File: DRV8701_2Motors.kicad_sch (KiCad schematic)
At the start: 24 parts, among them J1 Conn_01x02, J2 Conn_01x10, J3 Conn_01x10, SW1 SW_SPDT_321

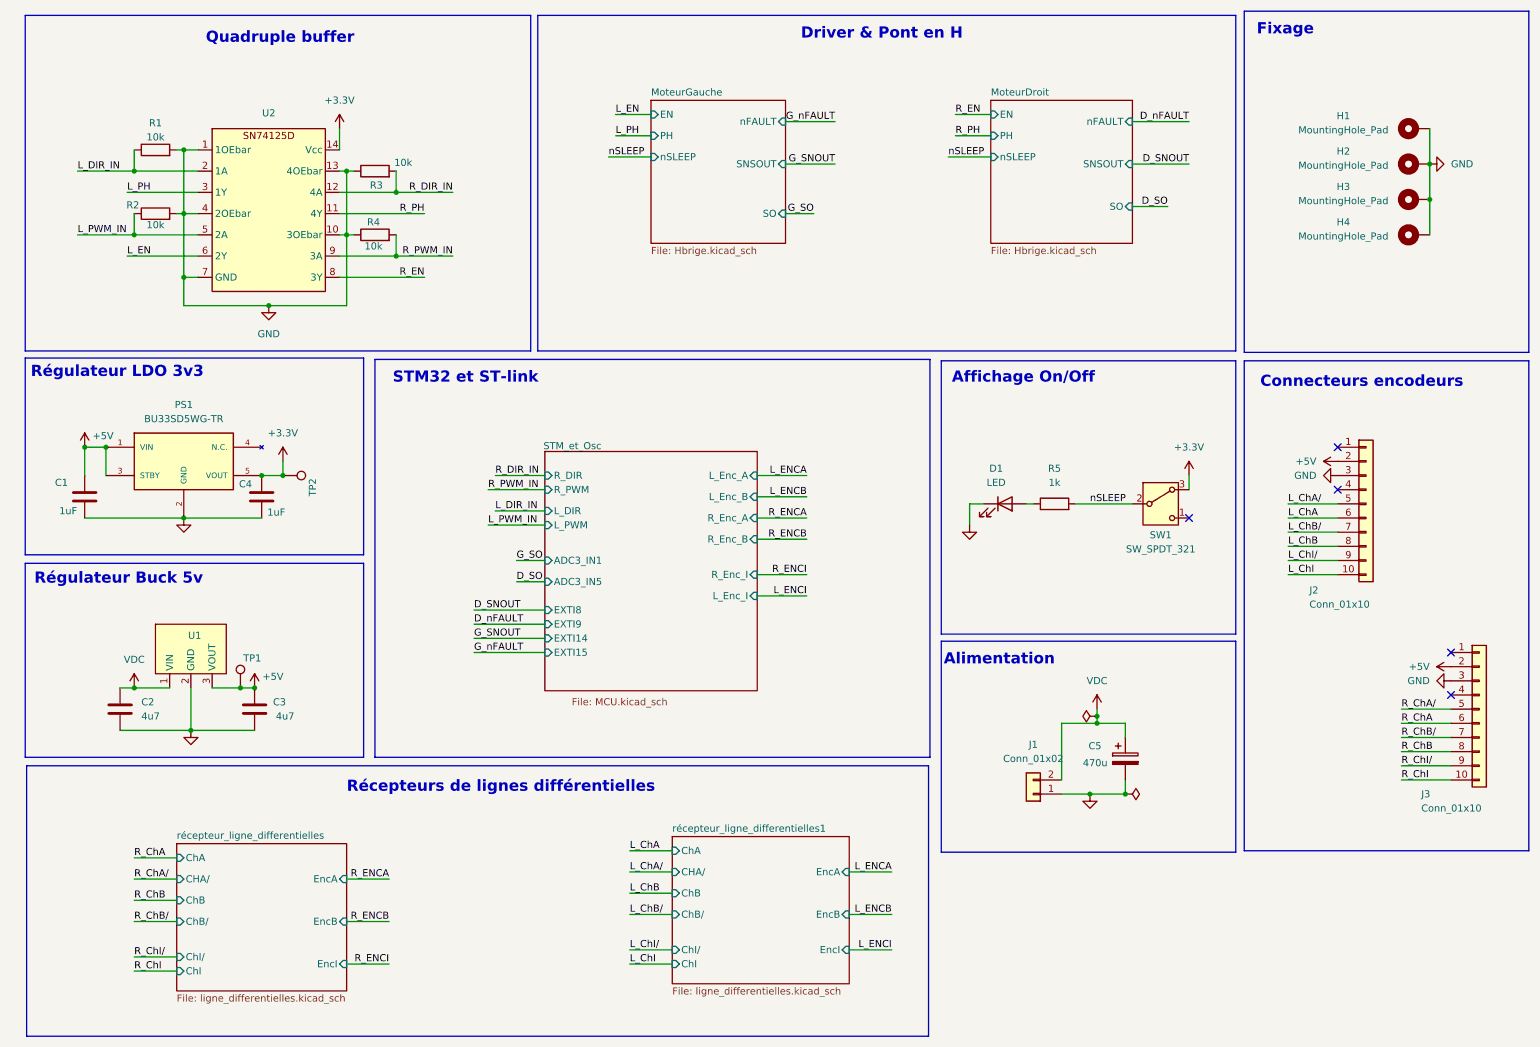
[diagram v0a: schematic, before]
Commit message: finalisation PCB
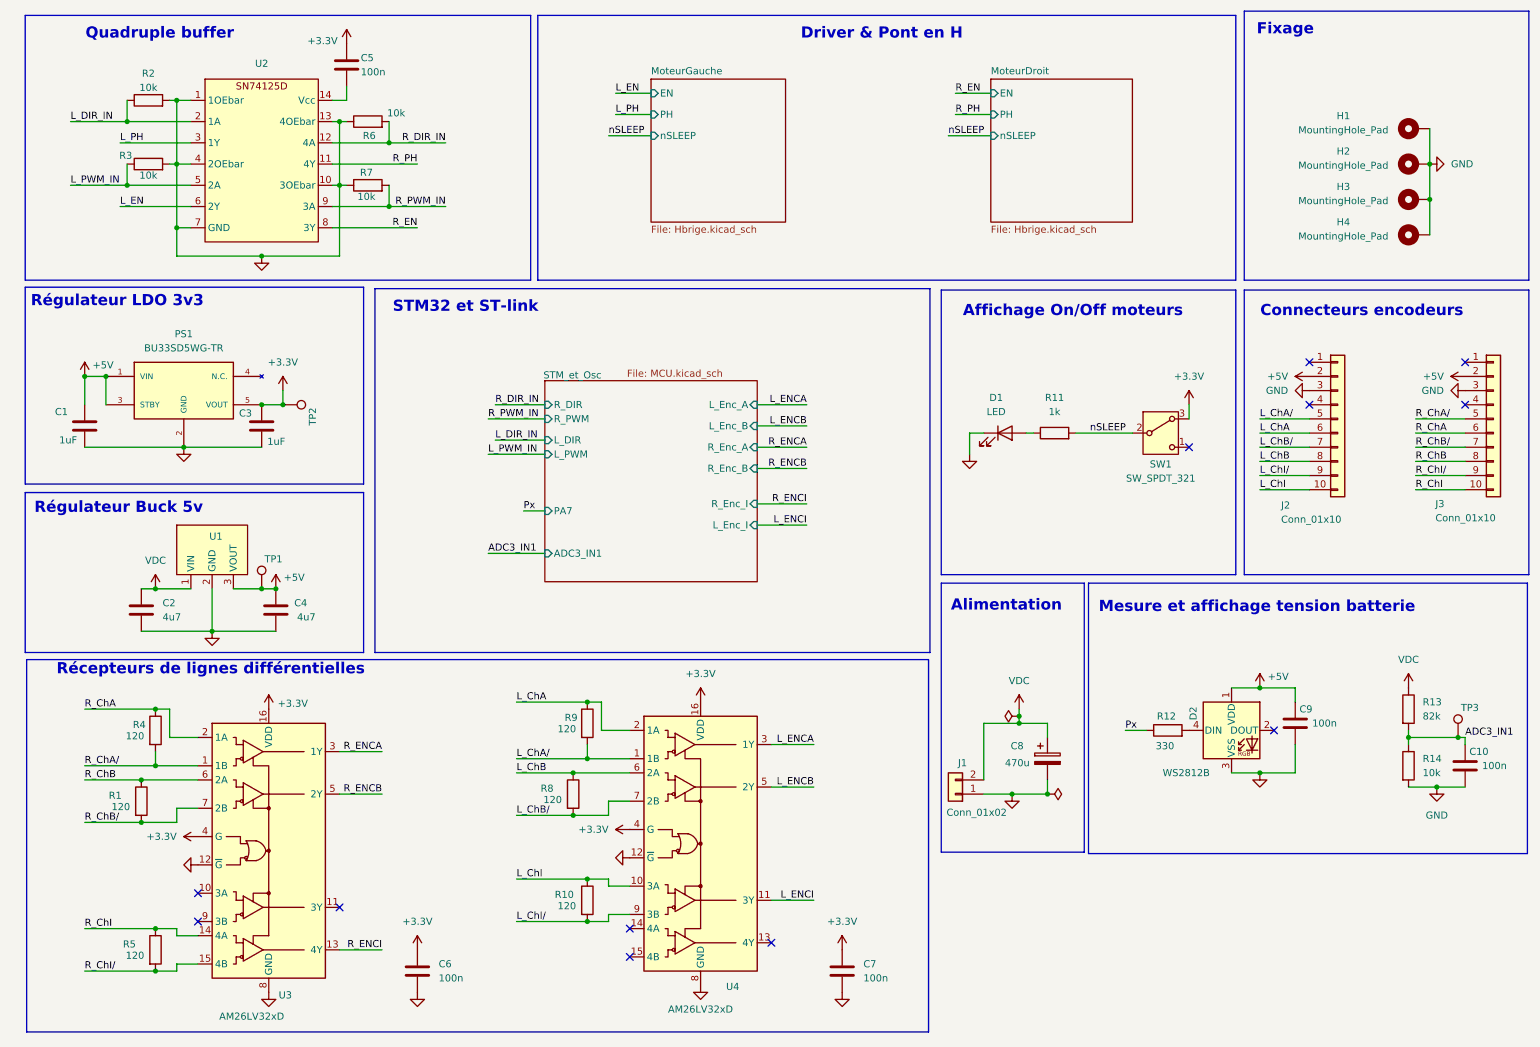
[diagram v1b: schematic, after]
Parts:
- added C10: 100n, Capacitor_SMD:C_0603_1608Metric_Pad1.08x0.95mm_HandSolder, symbol Device:C
- added C5, C6, C7, C9: 100n, Capacitor_SMD:C_0402_1005Metric, symbol Device:C
- added D2: WS2812B, LED_SMD:LED_WS2812B_PLCC4_5.0x5.0mm_P3.2mm, symbol LED:WS2812B
- added R1, R10, R4, R5, R8, R9: 120, Resistor_SMD:R_0201_0603Metric, symbol Device:R
- added R12: 330, Resistor_SMD:R_0603_1608Metric_Pad0.98x0.95mm_HandSolder, symbol Device:R
- added R13: 82k, Resistor_SMD:R_0603_1608Metric_Pad0.98x0.95mm_HandSolder, symbol Device:R
- added R14: 10k, Resistor_SMD:R_0603_1608Metric_Pad0.98x0.95mm_HandSolder, symbol Device:R
- added TP3: TestPoint, TestPoint:TestPoint_Pad_D1.5mm, symbol Connector:TestPoint
- added U3, U4: AM26LV32xD, Package_SO:SOIC-16_3.9x9.9mm_P1.27mm, symbol Interface:AM26LV32xD
- renumbered C4 to C3, C3 to C4, C5 to C8, R5 to R11, R1 to R2, R2 to R3, R3 to R6, R4 to R7
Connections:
- net +3.3V: now also C5.1, C6.1, C7.1, U3.16 (VDD), U3.4 (G), U4.16 (VDD), U4.4 (G); no longer U2.14 (Vcc)
- net +5V: now also C9.2, D2.1 (VDD)
- net GND: now also C10.1, C6.2, C7.2, C9.1, D2.3 (VSS), R14.2, U3.12 (~{G}), U3.8 (GND), U4.12 (~{G}), U4.8 (GND)
- net L_ChA: now also R9.1, U4.2 (1A)
- net L_ChA/: now also R9.2, U4.1 (1B)
- net L_ChB: now also R8.1, U4.6 (2A)
- net L_ChB/: now also R8.2, U4.7 (2B)
- net L_ChI: now also R10.1, U4.10 (3A)
- net L_ChI/: now also R10.2, U4.9 (3B)
- net L_ENCA: now also U4.3 (1Y)
- net L_ENCB: now also U4.5 (2Y)
- net L_ENCI: now also U4.11 (3Y)
- net R_ChA: now also R4.1, U3.2 (1A)
- net R_ChA/: now also R4.2, U3.1 (1B)
- net R_ChB: now also R1.1, U3.6 (2A)
- net R_ChB/: now also R1.2, U3.7 (2B)
- net R_ChI: now also R5.1, U3.14 (4A)
- net R_ChI/: now also R5.2, U3.15 (4B)
- net R_ENCA: now also U3.3 (1Y)
- net R_ENCB: now also U3.5 (2Y)
- net R_ENCI: now also U3.13 (4Y)
- net VDC: now also R13.1
- new net: D2.4 (DIN), R12.2
- new net: C5.2, U2.14 (Vcc)
- new net ADC3_IN1: C10.2, R13.2, R14.1, TP3.1
- new net Px: R12.1
- no-connect marks 5 -> 12
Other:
- removed sheet récepteur_ligne_differentielles
- removed sheet récepteur_ligne_differentielles1
- sheet MoteurDroit ports: added none; removed SNSOUT, SO, nFAULT
- sheet MoteurGauche ports: added none; removed SNSOUT, SO, nFAULT
- sheet STM_et_Osc ports: added PA7; removed ADC3_IN5, EXTI14, EXTI15, EXTI8, EXTI9
- note added: "Affichage On/Off moteurs"
- note added: "Mesure et affichage tension batterie"
- note removed: "Affichage On/Off"
- moved on the sheet: C1, C2, C3, C4, C8, D1, J1, J2, J3, PS1, R11, R2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
